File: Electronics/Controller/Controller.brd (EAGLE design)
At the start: 190 x 90 mm, 20 parts, among them Q1 IRFD9014, U1 GY-521MPU6050, X1 Battery, X2 Switch

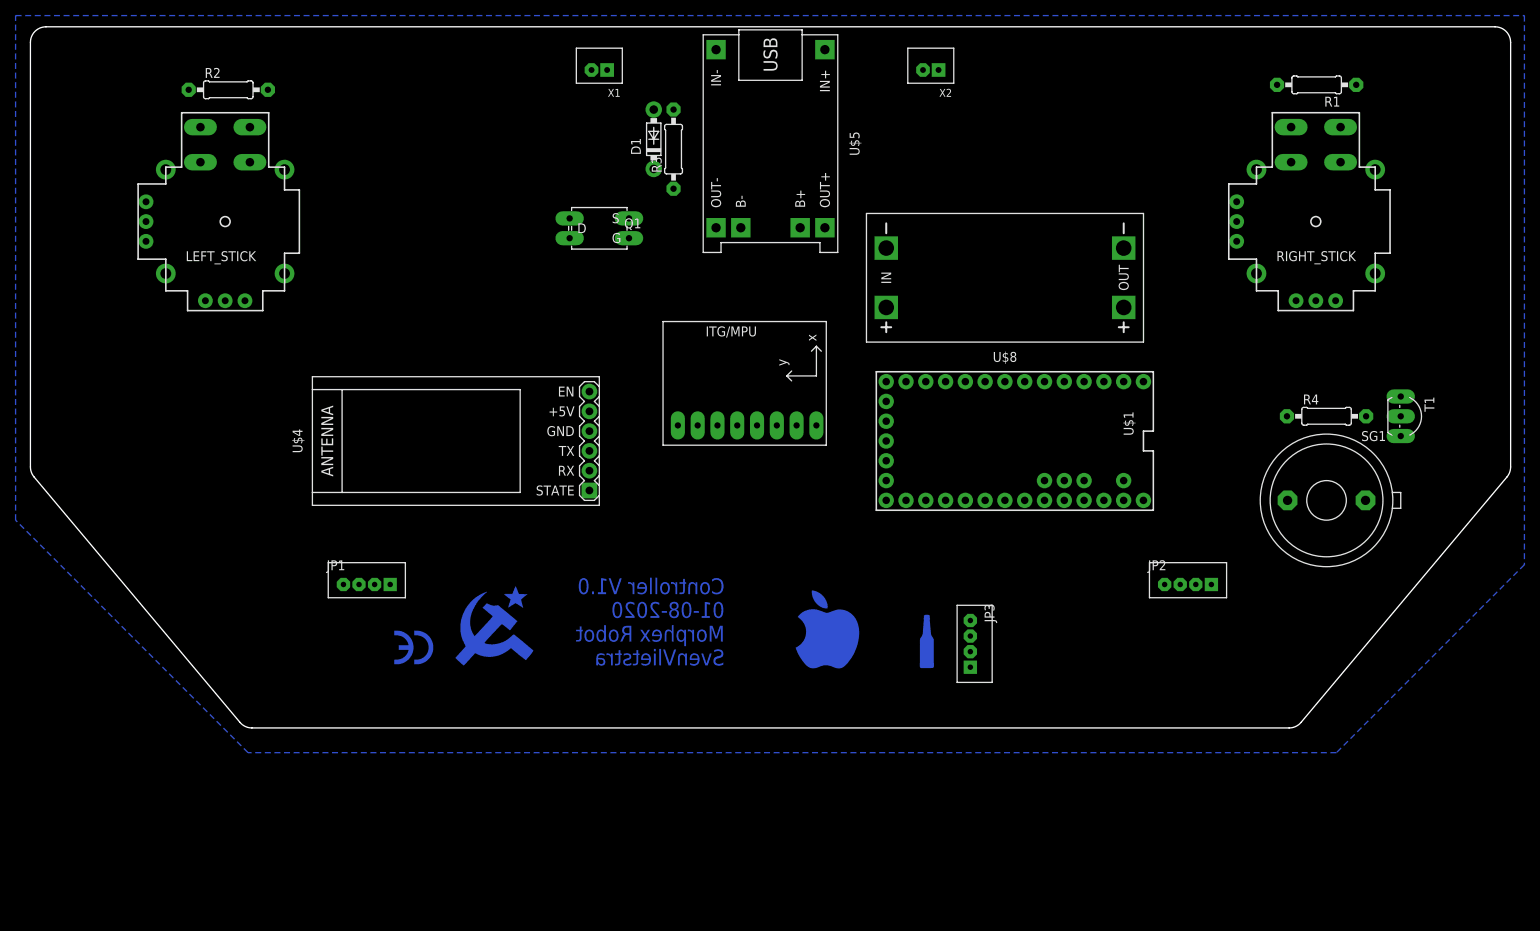
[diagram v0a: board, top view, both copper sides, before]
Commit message: .....
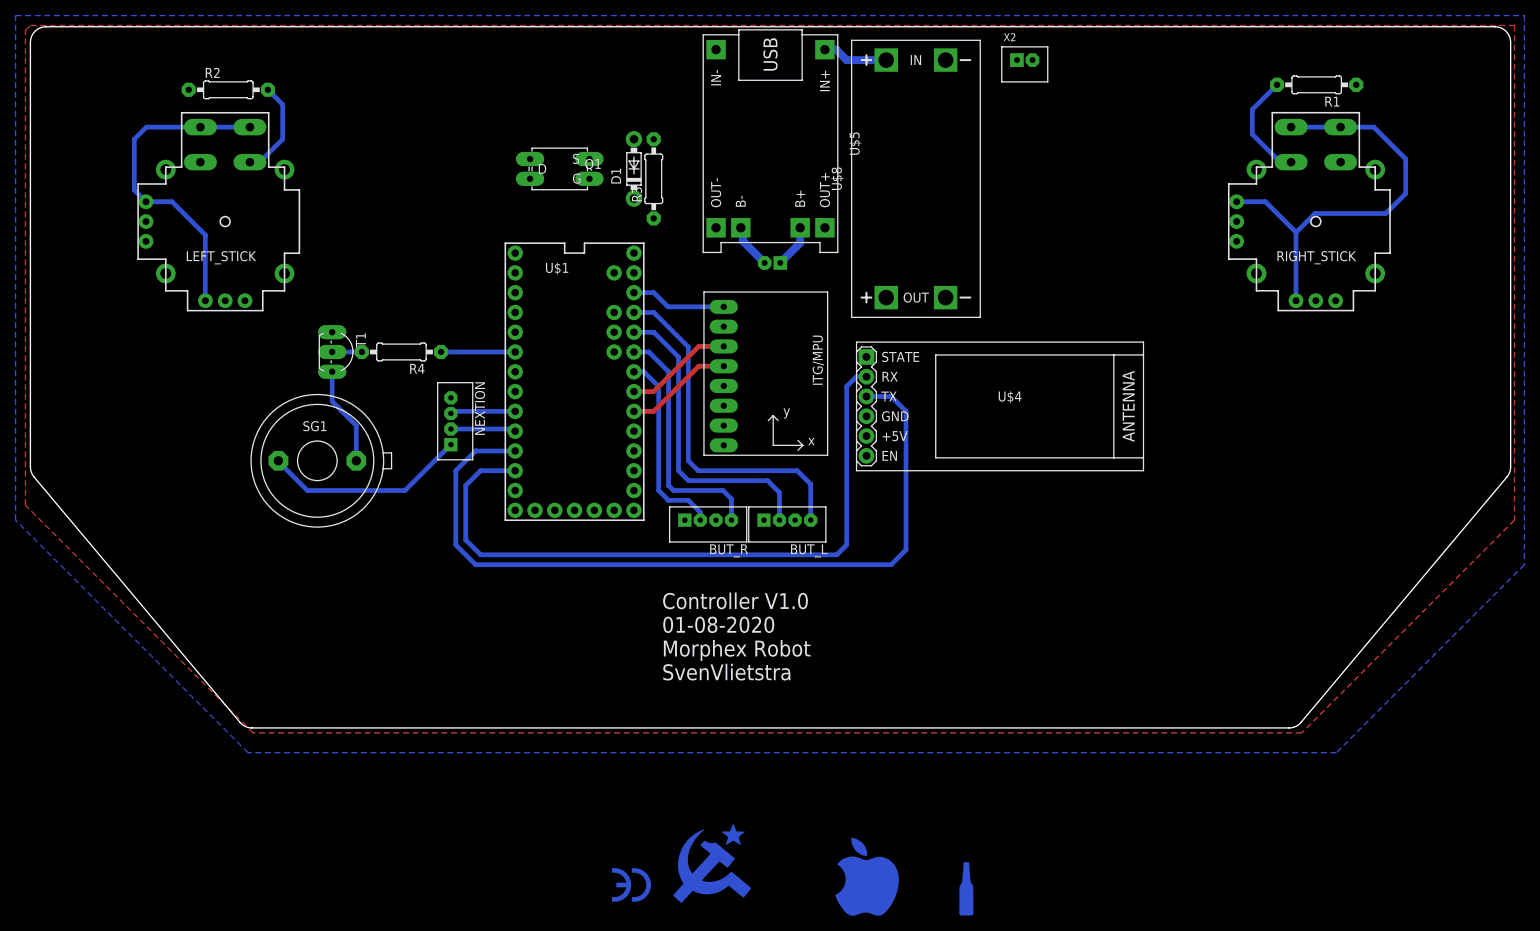
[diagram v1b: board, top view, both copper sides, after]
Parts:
- removed JP1, JP2, JP3: B4B-PH-K-S, con-JST PH:B4B-PH-K-S
- added BUT_L, BUT_R, NEXTION: B4B-PH-K-S, con-JST PH:B4B-PH-K-S
- moved T1 137.4 mm to (40.0, 48.3)
- moved SG1 129.6 mm to (36.8, 34.3)
- moved R4 119.0 mm to (47.6, 48.3), turned to 180 degrees
- moved U$4 70.0 mm to (124.5, 41.3), turned to 270 degrees
- moved U$1 57.0 mm to (69.8, 44.4), turned to 0 degrees
- moved X1 33.3 mm to (95.2, 59.7), flipped to the bottom, turned to 180 degrees
- moved U$8 17.1 mm to (113.7, 70.5), turned to 90 degrees
- moved X2 12.1 mm to (127.6, 85.7), turned to 180 degrees
- moved Q1 9.16 mm to (67.9, 71.8)
- moved U1 6.42 mm to (97.9, 45.2), turned to 0 degrees
- moved D1 4.58 mm to (77.5, 71.8)
- moved R3 4.58 mm to (80.0, 70.5)
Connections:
- net +3V3: now also BUT_L.1, BUT_L.3, BUT_R.1, BUT_R.3; no longer JP2.1, JP2.3, JP3.1, JP3.3
- net +5V: now also NEXTION.1; no longer JP1.1
- net BUT_1: now also BUT_L.2, U$1.22/A8; no longer JP2.2, U$1.20/A6
- net BUT_2: now also BUT_L.4, U$1.23/A9; no longer JP2.4, U$1.21/A7
- net BUT_3: now also BUT_R.2, U$1.20/A6; no longer JP3.2, U$1.22/A8
- net BUT_4: now also BUT_R.4, U$1.21/A7; no longer JP3.4, U$1.23/A9
- net GND: now also NEXTION.4; no longer JP1.4
- net NEX_RX: now also NEXTION.2; no longer JP1.2
- net NEX_TX: now also NEXTION.3; no longer JP1.3
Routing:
- net +3V3: track 0.00 -> 109.2 mm
- net BL_TX: track 0.00 -> 101.5 mm
- net BL_RX: track 0.00 -> 87.7 mm
- net BUT_2: track 0.00 -> 45.0 mm
- net BUT_1: track 0.00 -> 39.3 mm
- net +5V: track 0.00 -> 34.6 mm
- net BUT_4: track 0.00 -> 31.6 mm
- net SW1: track 0.00 -> 26.7 mm
- net BUT_3: track 0.00 -> 24.8 mm
- net GY_SDA: track 0.00 -> 13.9 mm
- net GY_SCL: track 0.00 -> 13.9 mm
- net N$8: track 0.00 -> 12.7 mm
- net BUZZER: track 0.00 -> 9.53 mm
- net NEX_RX: track 0.00 -> 8.37 mm
- net NEX_TX: track 0.00 -> 8.36 mm
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- added copper zone on layer 1, net GND
